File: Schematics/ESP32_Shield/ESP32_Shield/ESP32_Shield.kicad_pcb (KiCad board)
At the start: 2 copper layers, 27 x 50.2 mm, 19 parts, among them J1 Conn_01x10, Q1 Si1308EDL, Q4 Si2319CDS, U6 ADS1234IPW, U7 SHT30-DIS

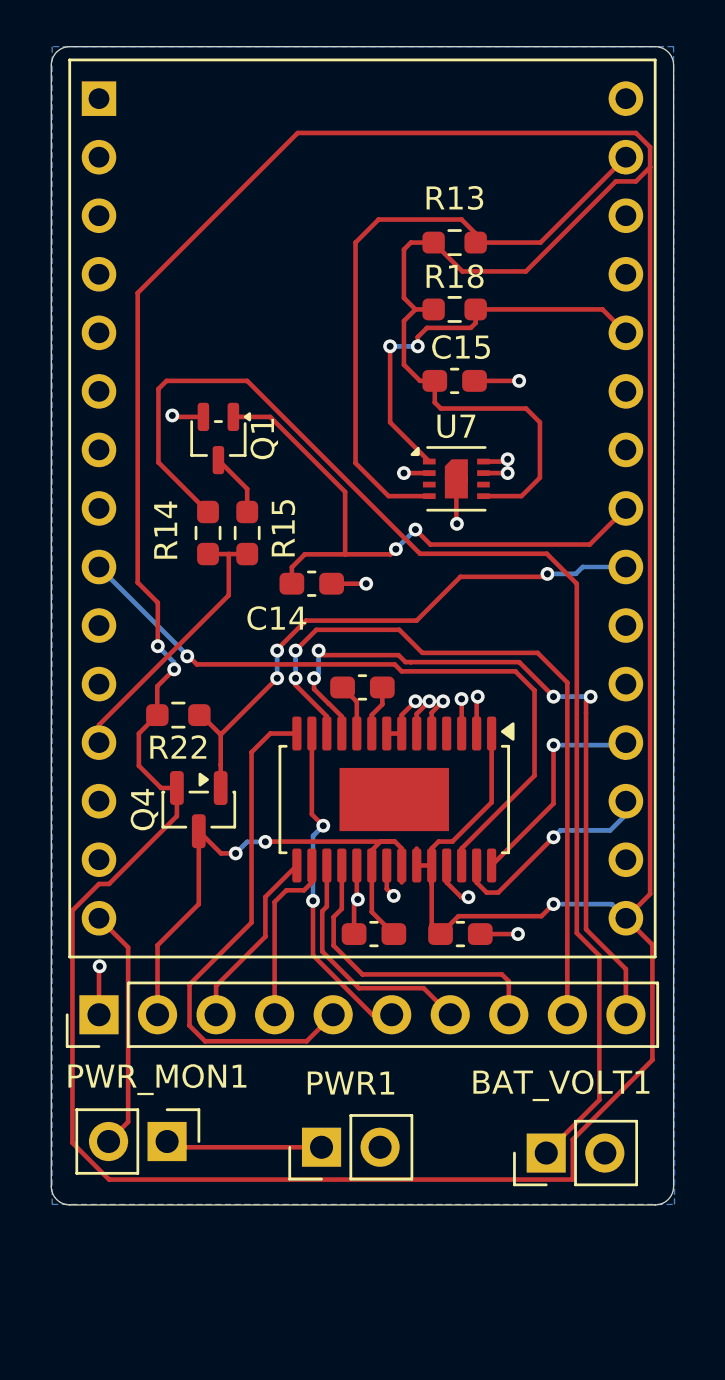
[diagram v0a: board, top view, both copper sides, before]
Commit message: Feedback umetzen
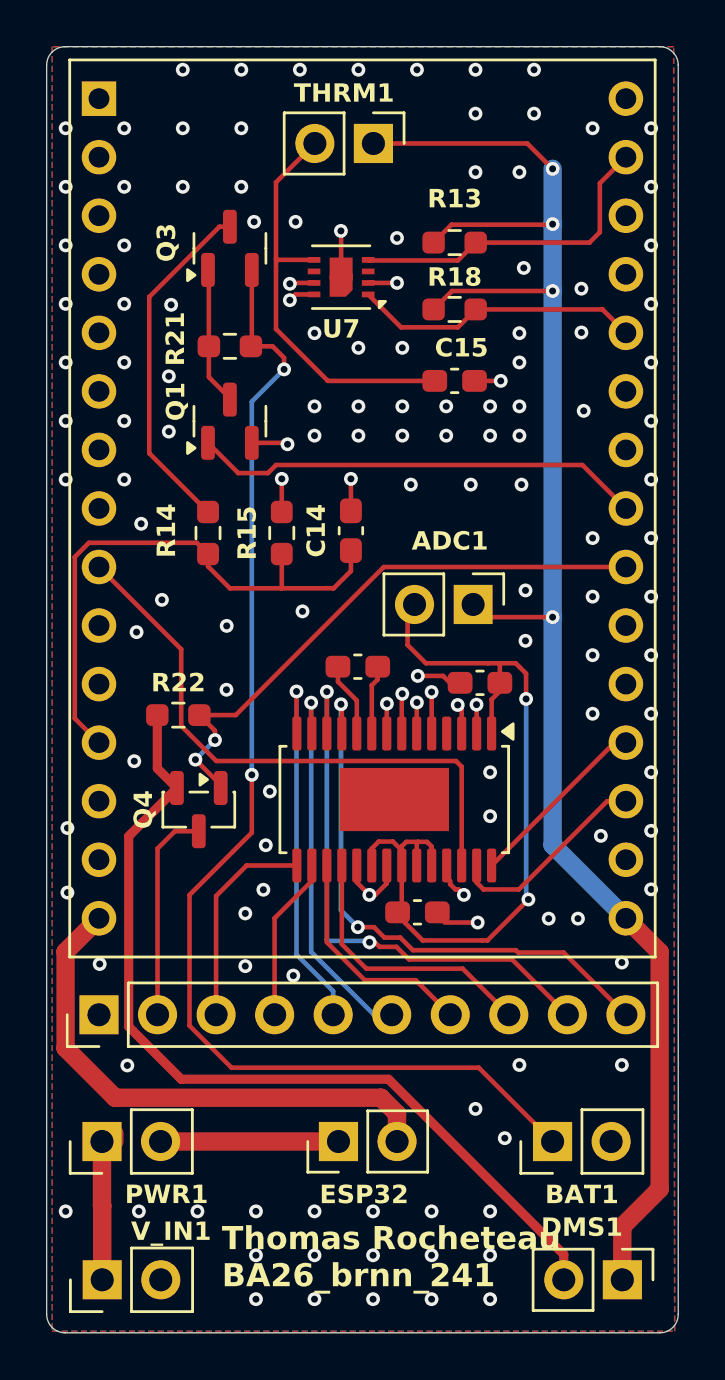
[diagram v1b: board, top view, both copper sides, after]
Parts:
- added ADC1: Conn_01x02, Connector_PinHeader_2.54mm:PinHeader_1x02_P2.54mm_Vertical, F.Cu at (128.8, 86.7)
- added DMS1: Conn_01x02, Connector_PinHeader_2.54mm:PinHeader_1x02_P2.54mm_Vertical, F.Cu at (135.3, 116.0)
- added ESP32: Conn_01x02, Connector_PinHeader_2.54mm:PinHeader_1x02_P2.54mm_Vertical, F.Cu at (123.0, 110.0)
- added Q3: Si2319CDS, Package_TO_SOT_SMD:SOT-23, F.Cu at (118.2, 71.2)
- added R21: 100k, Resistor_SMD:R_0603_1608Metric_Pad0.98x0.95mm_HandSolder, F.Cu at (118.2, 75.5)
- added THRM1: Conn_01x02, Connector_PinHeader_2.54mm:PinHeader_1x02_P2.54mm_Vertical, F.Cu at (124.5, 66.7)
- Q1: footprint Package_TO_SOT_SMD:SOT-323_SC-70 -> Package_TO_SOT_SMD:SOT-23
- moved V_IN1 11.1 mm to (112.7, 116.0)
- moved C1 10.9 mm to (129.1, 90.1), turned to 0 degrees
- moved U7 10.1 mm to (123.1, 72.5), turned to 180 degrees
- moved C14 2.86 mm to (123.5, 83.5), turned to -90 degrees
- moved PWR1 2.83 mm to (112.7, 110.0), turned to 90 degrees
- moved C13 2.11 mm to (126.4, 100.1), turned to 180 degrees
- moved R15 1.50 mm to (120.5, 83.6)
- moved C12 0.92 mm to (123.8, 89.4)
- moved Q1 0.90 mm to (118.2, 78.8), turned to 90 degrees
- moved BAT1 0.57 mm to (132.2, 110.0)
- renumbered BAT_VOLT1 to BAT1, PWR_MON1 to PWR1, PWR1 to V_IN1
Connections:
- C1 pad 2: +3.3V -> Net-(ADC1-Pin_2)
- C13 pad 2: Net-(J1-Pin_2) -> Net-(ADC1-Pin_2)
- C14 pad 2: en_meas -> bat_adc
- C15 pad 1: +3.3V -> Net-(THRM1-Pin_2)
- Q4 pad 2: +3.3V -> Net-(DMS1-Pin_2)
- R14 pad 1: +BATT -> Net-(Q3-D)
- R15 pad 1: Net-(Q1-D) -> GND
- R22 pad 2: +3.3V -> Net-(DMS1-Pin_2)
- U2 pad 15: +5V -> Net-(ESP32-Pin_2)
- U6 pad 1: +3.3V -> Net-(ADC1-Pin_2)
- U6 pad 20: Net-(J1-Pin_2) -> Net-(ADC1-Pin_2)
- U6 pad 22: Net-(J1-Pin_2) -> Net-(ADC1-Pin_2)
- U6 pad 23: +3.3V -> Net-(ADC1-Pin_2)
- U6 pad 24: +3.3V -> Net-(ADC1-Pin_2)
- U7 pad 5: +3.3V -> Net-(THRM1-Pin_2)
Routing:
- net +3.3V: track 190.1 -> 73.8 mm, vias 3 -> 4
- net Net-(DMS1-Pin_2): track 0.00 -> 38.8 mm
- net Net-(ADC1-Pin_2): track 0.00 -> 36.4 mm, vias 0 -> 2
- net Net-(ESP32-Pin_2): track 0.00 -> 23.0 mm
- net Net-(THRM1-Pin_2): track 0.00 -> 18.2 mm
- net Net-(J1-Pin_2): track 24.8 -> 9.31 mm, vias 2 -> 0
- net Net-(Q3-D): track 0.00 -> 15.1 mm
- net SCL: track 27.7 -> 14.3 mm
- net bat_adc: track 12.2 -> 24.5 mm
- net Net-(J1-Pin_9): track 31.8 -> 24.5 mm
- net Net-(J1-Pin_10): track 31.5 -> 24.5 mm, vias 4 -> 2
- net Net-(J1-Pin_5): track 22.8 -> 16.5 mm, vias 0 -> 1
- net en_meas: track 25.7 -> 19.6 mm, vias 2 -> 0
- net SDA: track 17.7 -> 12.5 mm, vias 2 -> 0
- net !PWDN: track 30.0 -> 25.6 mm, vias 1 -> 0
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- added copper zone on F.Cu, net GND
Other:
- board size 27 x 50.2 mm -> 27.4 x 55.8 mm
- board text added: "Thomas Rocheteau BA26_brnn_241"
